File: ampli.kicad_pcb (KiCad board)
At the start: 2 copper layers, 52 parts, among them J2 Conn_01x02, J3 Conn_01x03, K1 Relay_1CT, Q1 2N907, Q10 Q_PNP_BCE, Q11 BD138, Q12 Q_NPN_BCE, Q13 2N2222, Q2 2N907, Q3 2N907, Q4 2N2222, Q5 2N2222, Q6 2N907, Q7 2N907, Q8 BD139, Q9 BD139, U2 Jack_Mono

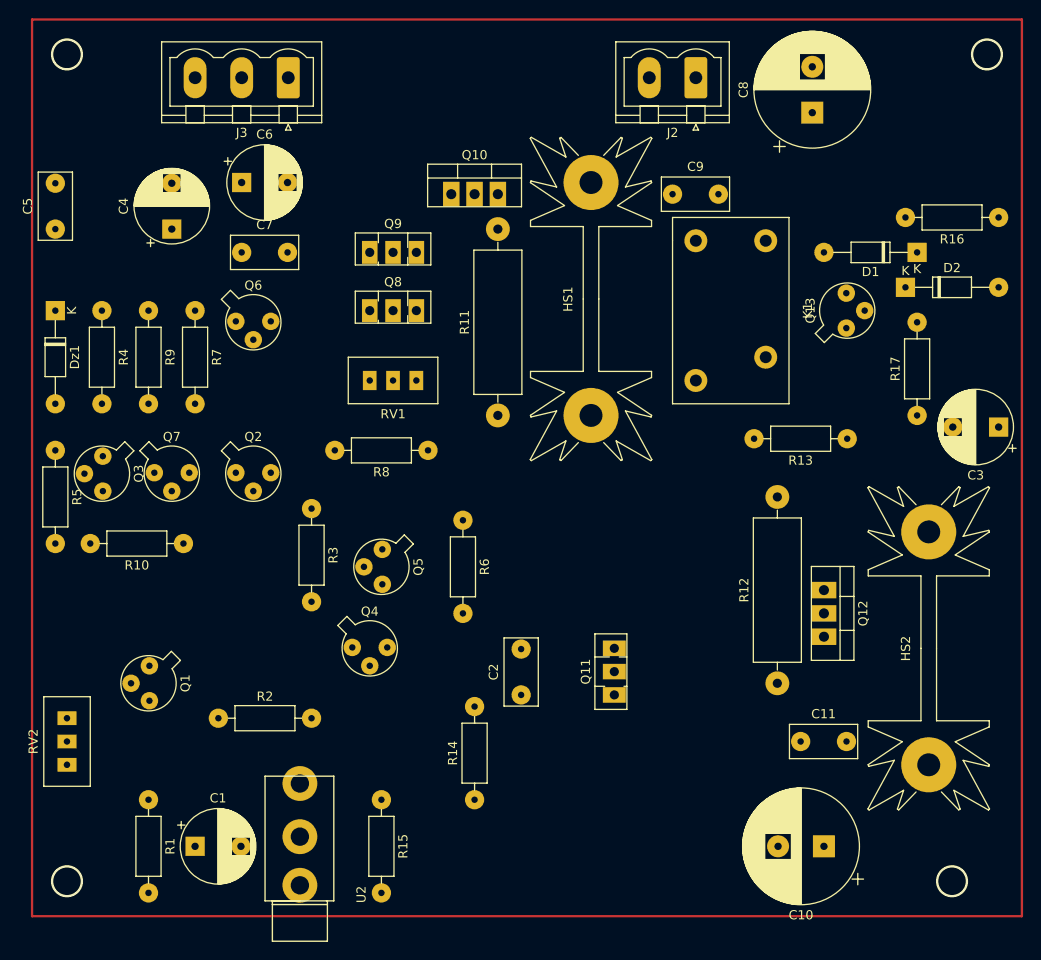
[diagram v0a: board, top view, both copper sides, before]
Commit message: pcb front
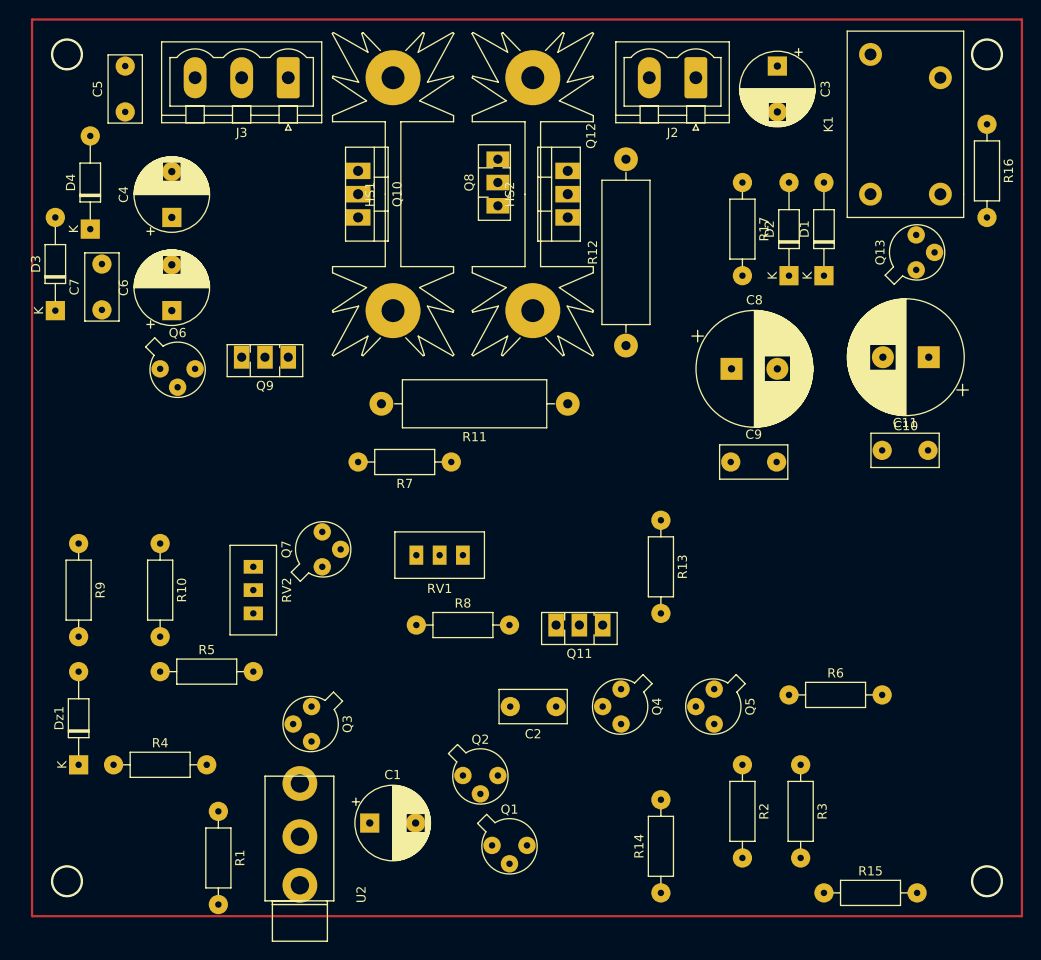
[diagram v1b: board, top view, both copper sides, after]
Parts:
- added D3: D, CmpAmpliAudio:D_DO-35_SOD27_P10.16mm_Horizontal, F.Cu at (74.9, 58.4)
- added D4: D, CmpAmpliAudio:D_DO-35_SOD27_P10.16mm_Horizontal, F.Cu at (78.7, 49.5)
- moved HS2 65.7 mm to (127.0, 45.7)
- moved R3 60.2 mm to (156.2, 108.0)
- moved R2 57.4 mm to (149.9, 108.0), turned to 270 degrees
- moved C10 54.6 mm to (170.2, 63.5)
- moved Dz1 49.6 mm to (77.5, 108.0), turned to 90 degrees
- moved R4 49.5 mm to (81.3, 108.0), turned to 0 degrees
- moved Q12 49.3 mm to (130.8, 48.3), turned to 90 degrees
- moved R15 49.3 mm to (158.8, 121.9), turned to 0 degrees
- moved C3 46.2 mm to (153.7, 31.8), turned to 270 degrees
- moved Q1 42.6 mm to (123.2, 116.8), turned to 0 degrees
- moved Q2 41.3 mm to (120.0, 109.2)
- moved R12 40.4 mm to (137.2, 62.2)
- moved R6 40.3 mm to (154.9, 100.3), turned to 0 degrees
- moved Q5 39.3 mm to (146.7, 100.3)
- moved Q3 35.5 mm to (102.8, 102.2)
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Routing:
- net -12V: track 0.00 -> 411.5 mm
- net (no net): track 411.5 -> 0.00 mm
